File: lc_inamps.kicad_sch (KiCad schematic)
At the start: 44 parts, among them J19 Conn_01x06_Female, J20 Conn_02x06_Odd_Even, U3 MCP6N11, U4 MCP6N11, U5 MCP6N11, U6 MCP6N11, U7 MCP6N11, U8 MCP6N11

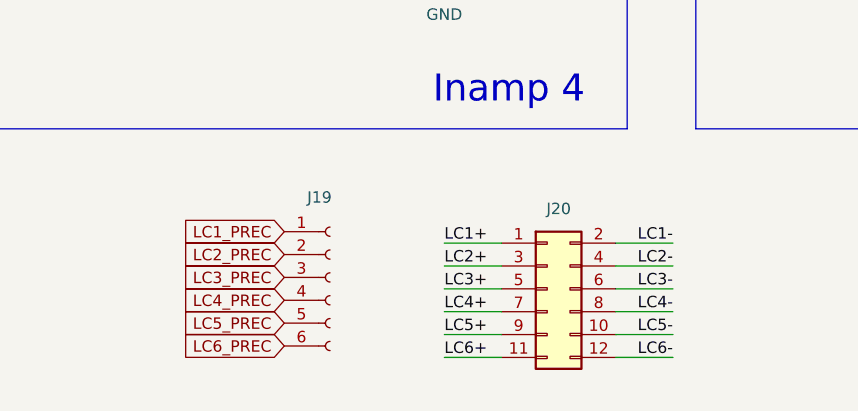
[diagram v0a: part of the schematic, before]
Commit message: complete arrangement for load cells
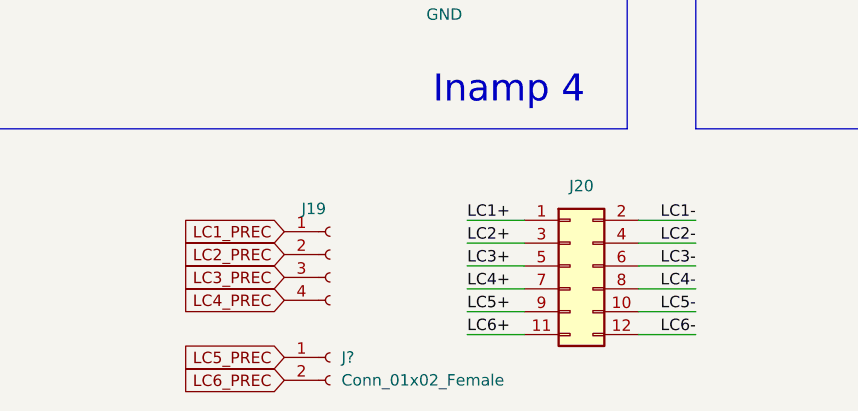
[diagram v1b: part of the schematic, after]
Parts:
- added J?: Conn_01x02_Female, Connector_PinHeader_2.54mm:PinHeader_1x02_P2.54mm_Vertical, symbol Connector:Conn_01x02_Female
- J19: symbol Connector:Conn_01x06_Female -> Connector:Conn_01x04_Female
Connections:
- net LC5_PREC: now also J?.1 (Pin_1); no longer J19.5 (Pin_5)
- net LC6_PREC: now also J?.2 (Pin_2); no longer J19.6 (Pin_6)
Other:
- moved on the sheet: J20
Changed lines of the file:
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@@
     (stroke (width 0) (type default) (color 0 0 0 0))
   )
-  (wire (pts (xy 109.22 176.53) (xy 102.87 176.53))
+  (wire (pts (xy 111.76 173.99) (xy 105.41 173.99))
     (stroke (width 0) (type default) (color 0 0 0 0))
   )
@@
     (stroke (width 0) (type default) (color 0 0 0 0))
   )
-  (wire (pts (xy 109.22 171.45) (xy 102.87 171.45))
+  (wire (pts (xy 111.76 168.91) (xy 105.41 168.91))
     (stroke (width 0) (type default) (color 0 0 0 0))
   )
@@
     (stroke (width 0) (type default) (color 0 0 0 0))
   )
-  (wire (pts (xy 83.82 168.91) (xy 90.17 168.91))
+  (wire (pts (xy 86.36 166.37) (xy 92.71 166.37))
     (stroke (width 0) (type default) (color 0 0 0 0))
   )
@@
     (stroke (width 0) (type default) (color 0 0 0 0))
   )
-  (wire (pts (xy 83.82 179.07) (xy 90.17 179.07))
+  (wire (pts (xy 86.36 176.53) (xy 92.71 176.53))
     (stroke (width 0) (type default) (color 0 0 0 0))
   )
@@
     (stroke (width 0) (type default) (color 0 0 0 0))
   )
-  (wire (pts (xy 109.22 168.91) (xy 102.87 168.91))
+  (wire (pts (xy 111.76 166.37) (xy 105.41 166.37))
     (stroke (width 0) (type default) (color 0 0 0 0))
   )
@@
     (stroke (width 0) (type default) (color 0 0 0 0))
   )
-  (wire (pts (xy 83.82 176.53) (xy 90.17 176.53))
+  (wire (pts (xy 86.36 173.99) (xy 92.71 173.99))
     (stroke (width 0) (type default) (color 0 0 0 0))
   )
@@
     (stroke (width 0) (type default) (color 0 0 0 0))
   )
-  (wire (pts (xy 109.22 173.99) (xy 102.87 173.99))
+  (wire (pts (xy 111.76 171.45) (xy 105.41 171.45))
     (stroke (width 0) (type default) (color 0 0 0 0))
   )
@@
     (stroke (width 0) (type default) (color 0 0 0 0))
   )
-  (wire (pts (xy 83.82 173.99) (xy 90.17 173.99))
+  (wire (pts (xy 86.36 171.45) (xy 92.71 171.45))
     (stroke (width 0) (type default) (color 0 0 0 0))
   )
@@
     (stroke (width 0) (type default) (color 0 0 0 0))
   )
-  (wire (pts (xy 83.82 171.45) (xy 90.17 171.45))
+  (wire (pts (xy 86.36 168.91) (xy 92.71 168.91))
     (stroke (width 0) (type default) (color 0 0 0 0))
   )
@@
     (stroke (width 0) (type default) (color 0 0 0 0))
   )
-  (wire (pts (xy 83.82 166.37) (xy 90.17 166.37))
+  (wire (pts (xy 86.36 163.83) (xy 92.71 163.83))
     (stroke (width 0) (type default) (color 0 0 0 0))
   )
@@
     (stroke (width 0) (type default) (color 0 0 0 0))
   )
-  (wire (pts (xy 109.22 166.37) (xy 102.87 166.37))
+  (wire (pts (xy 111.76 163.83) (xy 105.41 163.83))
     (stroke (width 0) (type default) (color 0 0 0 0))
   )
@@
     (stroke (width 0) (type default) (color 0 0 0 0))
   )
-  (wire (pts (xy 109.22 179.07) (xy 102.87 179.07))
+  (wire (pts (xy 111.76 176.53) (xy 105.41 176.53))
     (stroke (width 0) (type default) (color 0 0 0 0))
   )
@@
     (effects (font (size 1.27 1.27)) (justify left bottom))
   )
-  (label "LC3+" (at 83.82 171.45 0)
+  (label "LC3+" (at 86.36 168.91 0)
     (effects (font (size 1.27 1.27)) (justify left bottom))
   )
@@
     (effects (font (size 1.27 1.27)) (justify left bottom))
   )
-  (label "LC6+" (at 83.82 179.07 0)
+  (label "LC6+" (at 86.36 176.53 0)
     (effects (font (size 1.27 1.27)) (justify left bottom))
   )
-  (label "LC5+" (at 83.82 176.53 0)
+  (label "LC5+" (at 86.36 173.99 0)
     (effects (font (size 1.27 1.27)) (justify left bottom))
   )
@@
     (effects (font (size 1.27 1.27)) (justify left bottom))
   )
-  (label "LC3-" (at 109.22 171.45 180)
+  (label "LC3-" (at 111.76 168.91 180)
     (effects (font (size 1.27 1.27)) (justify right bottom))
   )
@@
     (effects (font (size 1.27 1.27)) (justify left bottom))
   )
-  (label "LC1-" (at 109.22 166.37 180)
+  (label "LC1-" (at 111.76 163.83 180)
     (effects (font (size 1.27 1.27)) (justify right bottom))
   )
@@
     (effects (font (size 1.27 1.27)) (justify left bottom))
   )
-  (label "LC2+" (at 83.82 168.91 0)
+  (label "LC2+" (at 86.36 166.37 0)
     (effects (font (size 1.27 1.27)) (justify left bottom))
   )
-  (label "LC5-" (at 109.22 176.53 180)
+  (label "LC5-" (at 111.76 173.99 180)
     (effects (font (size 1.27 1.27)) (justify right bottom))
   )
-  (label "LC4-" (at 109.22 173.99 180)
+  (label "LC4-" (at 111.76 171.45 180)
     (effects (font (size 1.27 1.27)) (justify right bottom))
   )
@@
     (effects (font (size 1.27 1.27)) (justify left bottom))
   )
-  (label "LC2-" (at 109.22 168.91 180)
+  (label "LC2-" (at 111.76 166.37 180)
     (effects (font (size 1.27 1.27)) (justify right bottom))
   )
@@
     (effects (font (size 1.27 1.27)) (justify left bottom))
   )
-  (label "LC6-" (at 109.22 179.07 180)
+  (label "LC6-" (at 111.76 176.53 180)
     (effects (font (size 1.27 1.27)) (justify right bottom))
   )
@@
     (effects (font (size 1.27 1.27)) (justify left bottom))
   )
-  (label "LC4+" (at 83.82 173.99 0)
+  (label "LC4+" (at 86.36 171.45 0)
     (effects (font (size 1.27 1.27)) (justify left bottom))
   )
-  (label "LC1+" (at 83.82 166.37 0)
+  (label "LC1+" (at 86.36 163.83 0)
     (effects (font (size 1.27 1.27)) (justify left bottom))
   )
@@
     )
   )
-  (global_label "LC6_PREC" (shape input) (at 66.04 177.8 180) (fields_autoplaced)
+  (global_label "LC6_PREC" (shape input) (at 66.04 181.61 180) (fields_autoplaced)
     (effects (font (size 1.27 1.27)) (justify right))
-    (property "Intersheet References" "${INTERSHEET_REFS}" (id 0) (at 54.1926 177.7206 0)
+    (property "Intersheet References" "${INTERSHEET_REFS}" (id 0) (at 54.1926 181.5306 0)
       (effects (font (size 1.27 1.27)) (justify right) hide)
     )
   )
-  (global_label "LC5_PREC" (shape input) (at 66.04 175.26 180) (fields_autoplaced)
+  (global_label "LC5_PREC" (shape input) (at 66.04 179.07 180) (fields_autoplaced)
     (effects (font (size 1.27 1.27)) (justify right))
-    (property "Intersheet References" "${INTERSHEET_REFS}" (id 0) (at 54.1926 175.1806 0)
+    (property "Intersheet References" "${INTERSHEET_REFS}" (id 0) (at 54.1926 178.9906 0)
       (effects (font (size 1.27 1.27)) (justify right) hide)
     )
@@
     (pin "1")
   )
-  (symbol (lib_id "Connector:Conn_01x06_Female") (at 71.12 170.18 0) (unit 1)
-    (in_bom yes) (on_board yes)
-    (property "Reference" "J19" (id 0) (at 68.58 161.29 0)
-      (effects (font (size 1.27 1.27)) (justify left))
-    )
-    (property "Value" "Conn_01x06_Female" (id 1) (at 72.39 171.4499 0)
+  (symbol (lib_id "Connector:Conn_01x04_Female") (at 71.12 167.64 0) (unit 1)
+    (in_bom yes) (on_board yes)
+    (property "Reference" "J19" (id 0) (at 67.945 162.56 0)
+      (effects (font (size 1.27 1.27)) (justify left))
+    )
+    (property "Value" "Conn_01x06_Female" (id 1) (at 72.39 168.9099 0)
       (effects (font (size 1.27 1.27)) (justify left) hide)
     )
-    (property "Footprint" "Connector_PinSocket_2.54mm:PinSocket_1x06_P2.54mm_Vertical" (id 2) (at 71.12 170.18 0)
-      (effects (font (size 1.27 1.27)) hide)
-    )
-    (property "Datasheet" "~" (id 3) (at 71.12 170.18 0)
+    (property "Footprint" "Connector_PinSocket_2.54mm:PinSocket_1x06_P2.54mm_Vertical" (id 2) (at 71.12 167.64 0)
+      (effects (font (size 1.27 1.27)) hide)
+    )
+    (property "Datasheet" "~" (id 3) (at 71.12 167.64 0)
       (effects (font (size 1.27 1.27)) hide)
     )
@@
     (pin "3")
     (pin "4")
-    (pin "5")
-    (pin "6")
   )
   (symbol (lib_id "power:+5V") (at 212.09 110.49 0) (unit 1)
@@
     (pin "1")
   )
-  (symbol (lib_id "Connector_Generic:Conn_02x06_Odd_Even") (at 95.25 171.45 0) (unit 1)
-    (in_bom yes) (on_board yes) (fields_autoplaced)
-    (property "Reference" "J20" (id 0) (at 96.52 162.56 0))
-    (property "Value" "Conn_02x06_Odd_Even" (id 1) (at 96.52 162.56 0)
-      (effects (font (size 1.27 1.27)) hide)
-    )
-    (property "Footprint" "Connector_PinSocket_2.54mm:PinSocket_2x06_P2.54mm_Vertical" (id 2) (at 95.25 171.45 0)
-      (effects (font (size 1.27 1.27)) hide)
-    )
-    (property "Datasheet" "~" (id 3) (at 95.25 171.45 0)
+  (symbol (lib_id "Connector_Generic:Conn_02x06_Odd_Even") (at 97.79 168.91 0) (unit 1)
+    (in_bom yes) (on_board yes) (fields_autoplaced)
+    (property "Reference" "J20" (id 0) (at 99.06 160.02 0))
+    (property "Value" "Conn_02x06_Odd_Even" (id 1) (at 99.06 160.02 0)
+      (effects (font (size 1.27 1.27)) hide)
+    )
+    (property "Footprint" "Connector_PinSocket_2.54mm:PinSocket_2x06_P2.54mm_Vertical" (id 2) (at 97.79 168.91 0)
+      (effects (font (size 1.27 1.27)) hide)
+    )
+    (property "Datasheet" "~" (id 3) (at 97.79 168.91 0)
       (effects (font (size 1.27 1.27)) hide)
     )
@@
     (pin "1")
   )
+  (symbol (lib_id "Connector:Conn_01x02_Female") (at 71.12 179.07 0) (unit 1)
+    (in_bom yes) (on_board yes) (fields_autoplaced)
+    (property "Reference" "J?" (id 0) (at 72.39 179.0699 0)
+      (effects (font (size 1.27 1.27)) (justify left))
+    )
+    (property "Value" "Conn_01x02_Female" (id 1) (at 72.39 181.6099 0)
+      (effects (font (size 1.27 1.27)) (justify left))
+    )
+    (property "Footprint" "Connector_PinHeader_2.54mm:PinHeader_1x02_P2.54mm_Vertical" (id 2) (at 71.12 179.07 0)
+      (effects (font (size 1.27 1.27)) hide)
+    )
+    (property "Datasheet" "~" (id 3) (at 71.12 179.07 0)
+      (effects (font (size 1.27 1.27)) hide)
+    )
+    (pin "1")
+    (pin "2")
+  )
   (symbol (lib_id "Device:Fuse") (at 36.83 114.3 0) (unit 1)
